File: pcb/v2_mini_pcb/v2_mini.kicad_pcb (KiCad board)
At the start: 6 copper layers, 60.8 x 35.1 mm, 118 parts, among them J1 Conn_Coaxial, J2 GTFP08441BEU, J3 SFV24R-2STE1HLF, J5 TC2030, J6 USB4105-GF-A, Q1 NTNS3164NZT5G, SW1 SW_Push, SW2 SW_Push, SW3 SW_Push, SW4 SW_Push, SW5 SW_Push, SW6 SW_Push, SW7 SW_Push, U1 UM980, U10 TPS63802DLAR, U3 SCH16T-K01-1, U4 LP5813ADRRR, U5 TCA9536ADTMR, U6 TPD4EUSB30, U7 MAX16169AALTA+T, U8 BQ25622ERYKR, U9 MAX17048G_T10

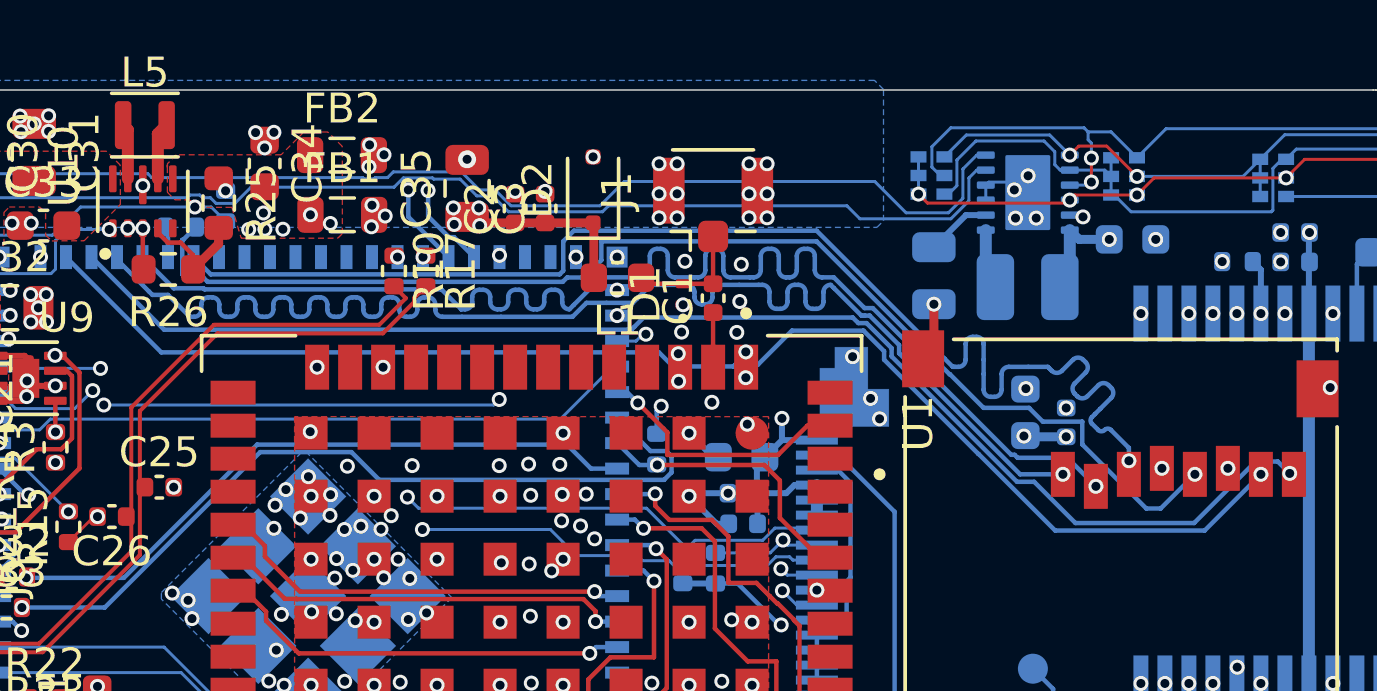
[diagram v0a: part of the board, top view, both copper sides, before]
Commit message: better length tuning
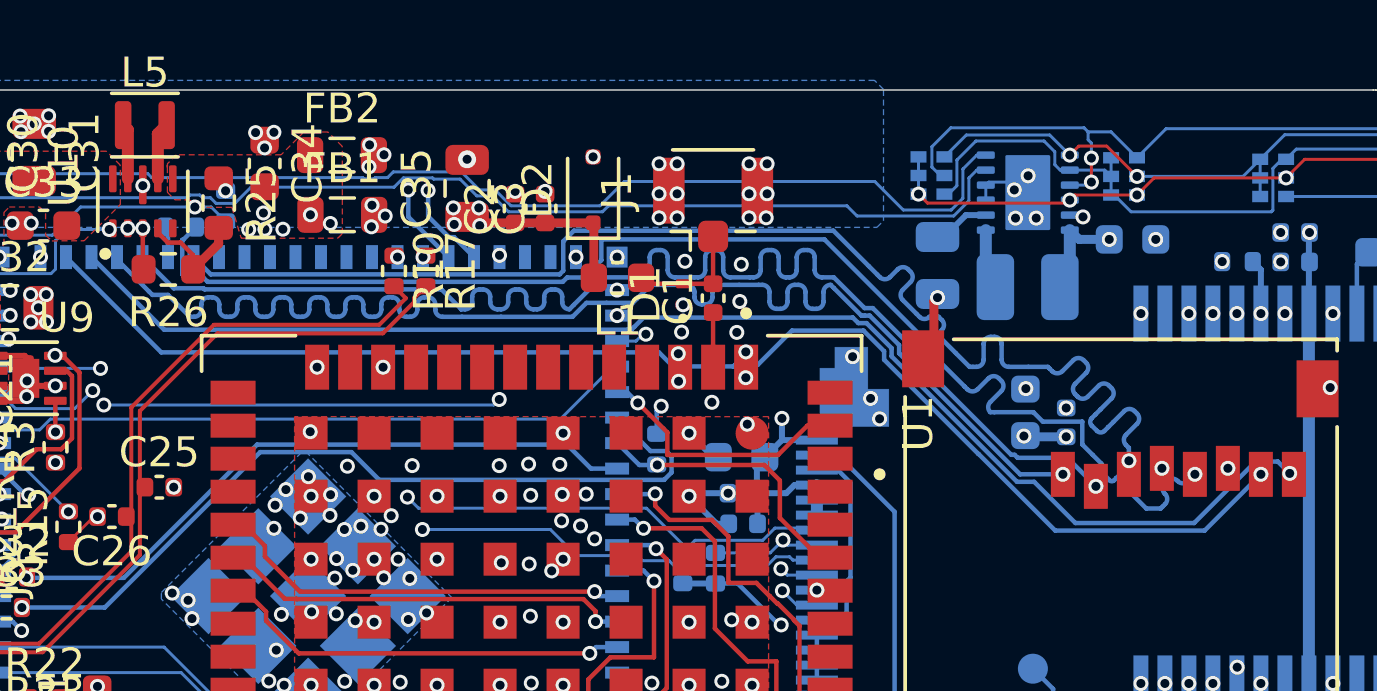
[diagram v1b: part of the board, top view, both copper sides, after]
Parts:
- moved C28 0.36 mm to (118.7, 84.5)
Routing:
- net Net-(J2-CLK): track 41.2 -> 44.2 mm
- net /ESP32-S31 MCU/SD_CMD: track 42.9 -> 44.7 mm
